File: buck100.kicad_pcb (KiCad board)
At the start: 2 copper layers, 10.5 x 19.5 mm, 15 parts, among them J1 Conn_01x03_Male, U2 LM5163DDAR

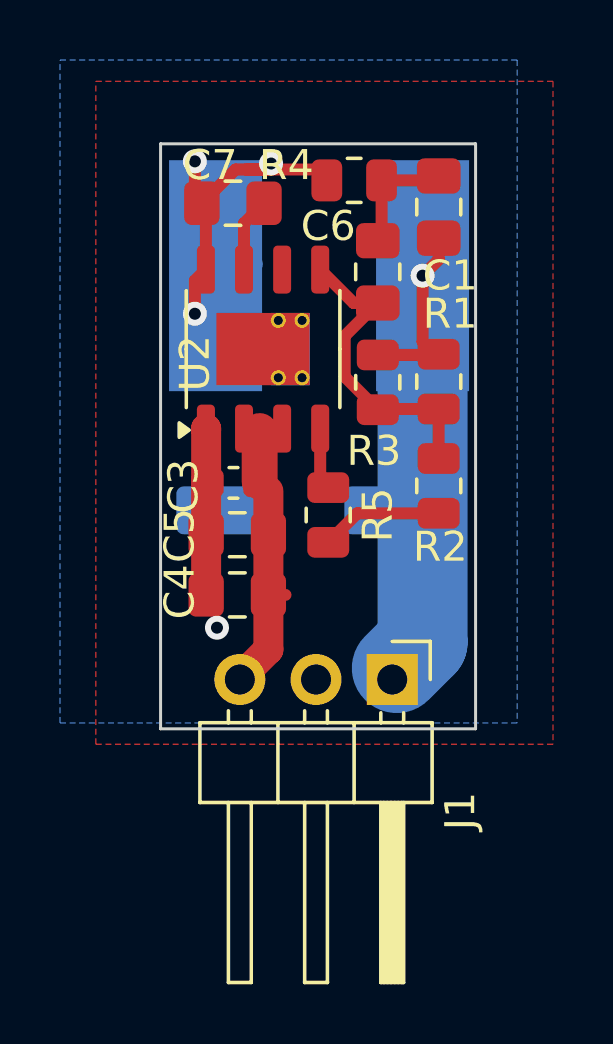
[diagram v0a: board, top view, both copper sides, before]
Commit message: docs, vias
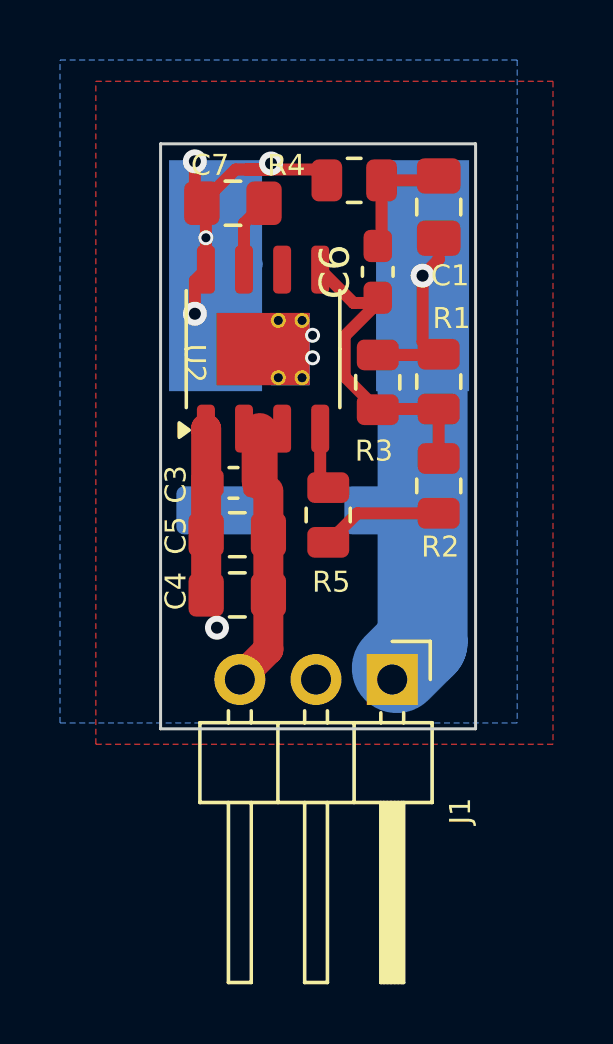
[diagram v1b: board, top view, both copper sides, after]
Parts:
- C1: value ~ -> 2200 pF, 100 V
- C6: value ~ -> 56pF, 50V; footprint Capacitor_SMD:C_0805_2012Metric_Pad1.18x1.45mm_HandSolder -> Capacitor_SMD:C_0603_1608Metric_Pad1.08x0.95mm_HandSolder
- C7: value 2200 pF, 50 V, X7R, 10% -> 2200 pF, 50 V
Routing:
- net VIN: track 9.31 -> 8.74 mm
- net SW: vias 3 -> 4
- net GND: vias 1 -> 3
